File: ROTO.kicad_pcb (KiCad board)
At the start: 2 copper layers, 7 parts, among them J1 POWER INPUT, J2 RELAY, J3 Switch, U1 LM7805, U2 SX1509

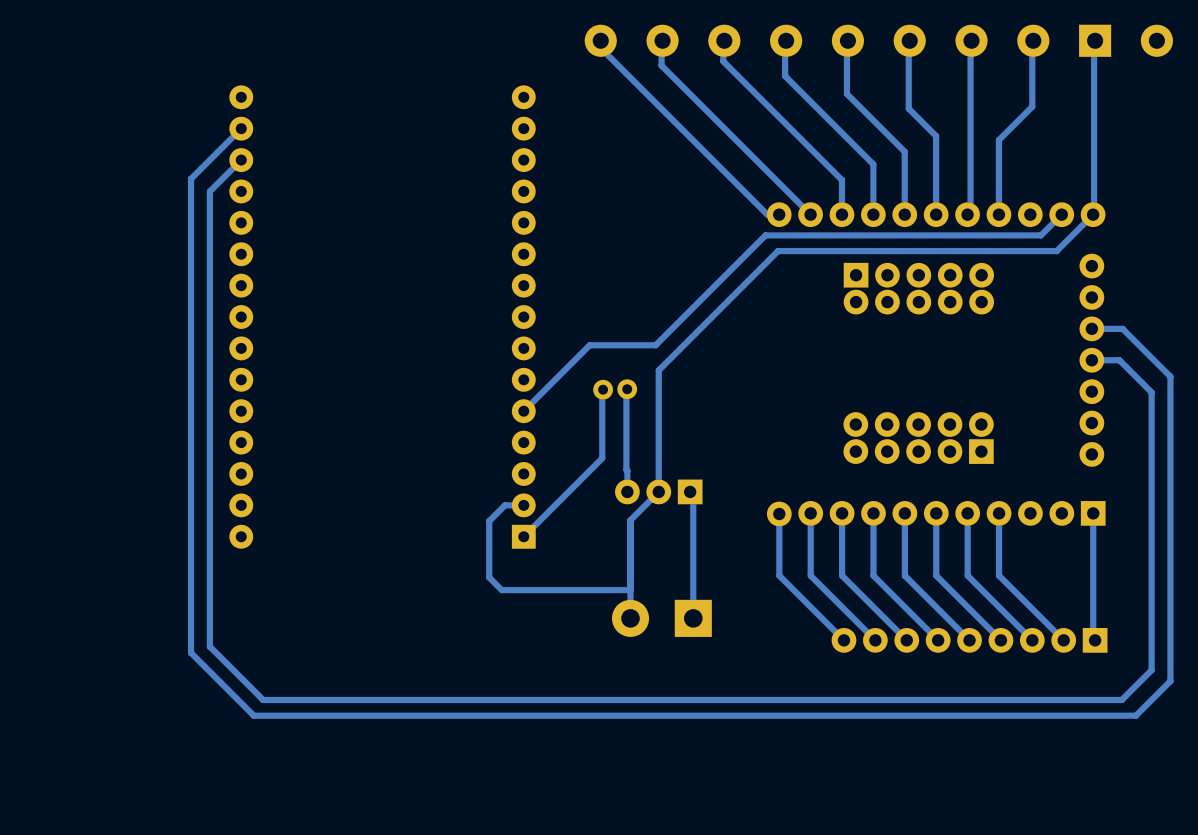
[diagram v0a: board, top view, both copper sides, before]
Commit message: Updated PDF
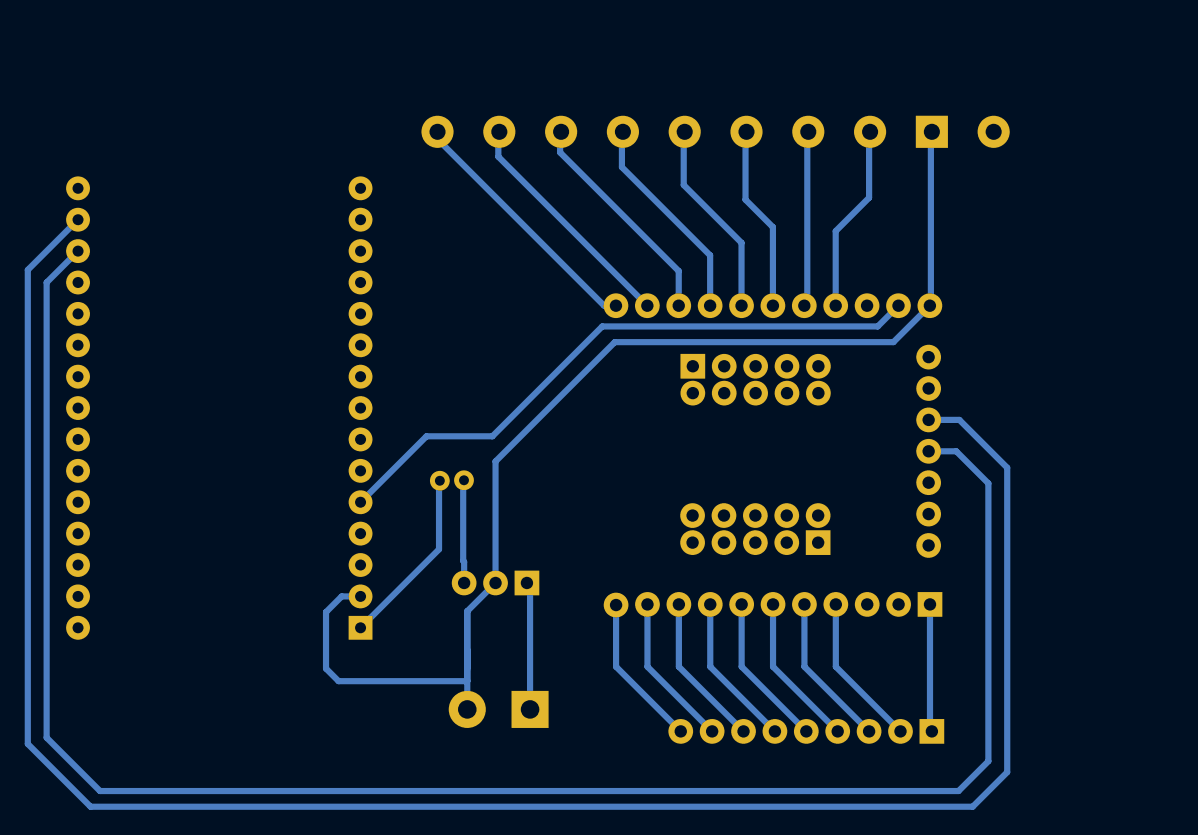
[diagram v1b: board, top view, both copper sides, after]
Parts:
- moved A1 15.1 mm to (114.6, 97.5)
- moved C1 15.1 mm to (134.1, 103.4)
- moved J1 15.1 mm to (139.7, 121.9)
- moved J2 15.1 mm to (151.9, 123.7)
- moved J3 15.1 mm to (177.2, 75.2)
- moved U1 15.1 mm to (139.4, 111.7)
- moved U2 15.1 mm to (159.1, 101.2)
